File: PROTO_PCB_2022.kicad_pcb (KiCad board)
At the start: 2 copper layers, 86.4 x 49.5 mm, 15 parts, among them J1 ECU_EN_CONNECTON_1, J2 SMALL_12V_BATTERY_CONNECTOR, J3 12V_EXTRA, J4 ECU_EN_CONECTION_2, J5 ECU_EN_CONECTION_3, K2 RT214012, Q1 HORN_MOSFET1, Q2 BRAKELIGHTS_MOSFET1

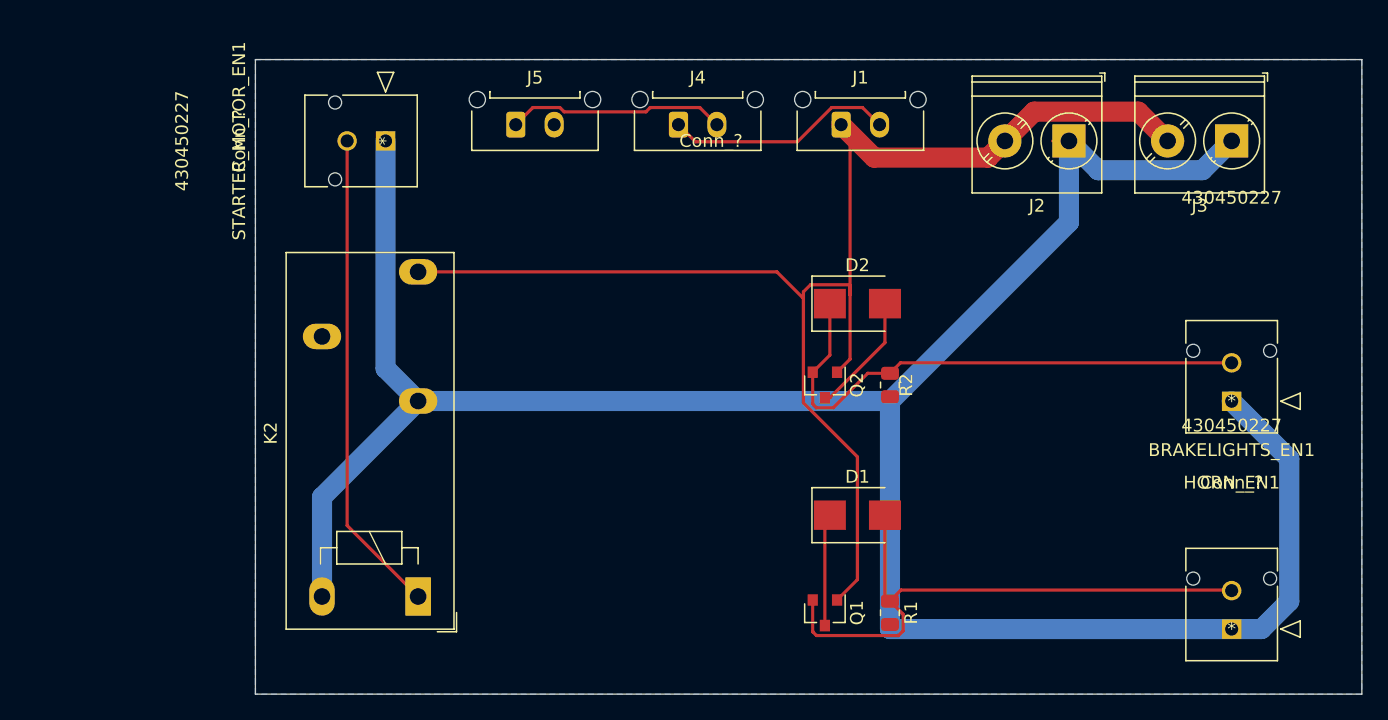
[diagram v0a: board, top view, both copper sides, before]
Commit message: Draft PCB for Report Purposes
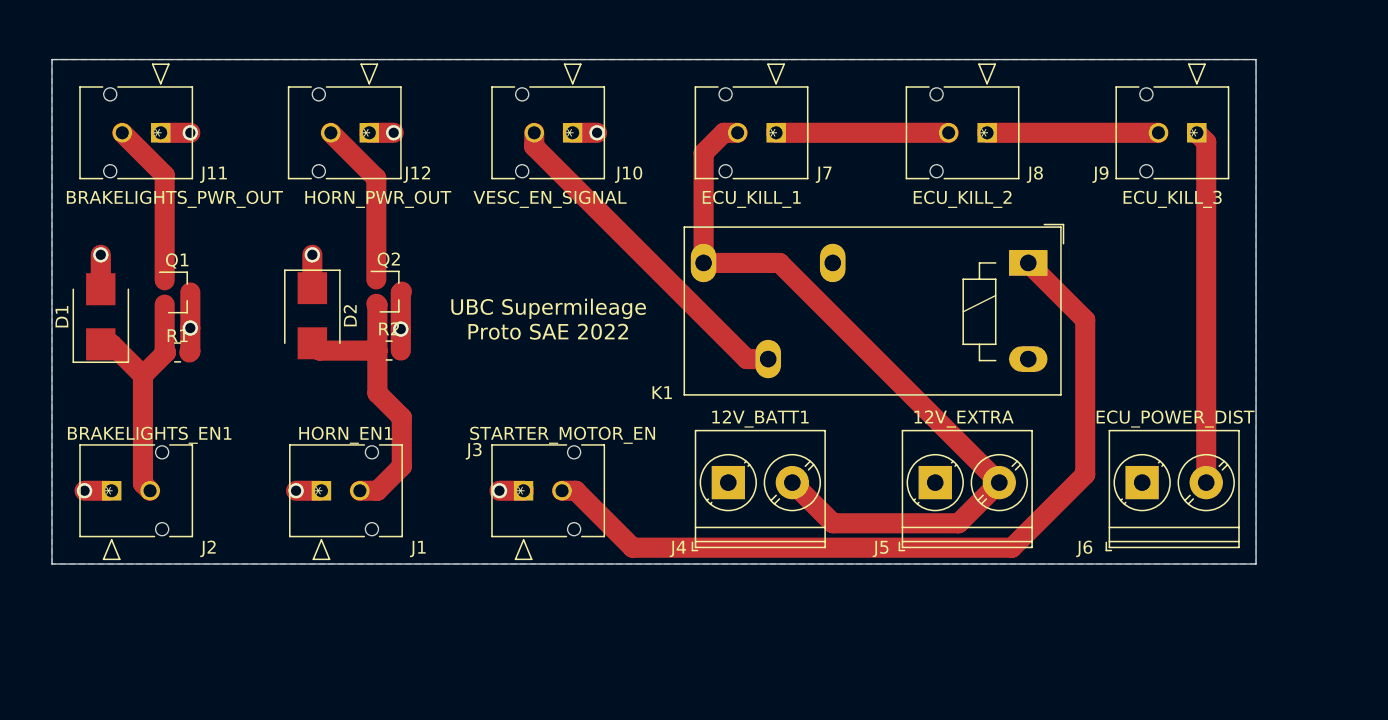
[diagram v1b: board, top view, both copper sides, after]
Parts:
- removed the J1 at (133.3, 83.8)
- removed the J4 at (120.7, 83.8)
- removed the J5 at (108.0, 83.8)
- added J10: VESC_EN_SIGNAL, Footprint Library:Molex_Proto_Microfit_Footprint, F.Cu at (112.4, 84.5)
- added J11: BRAKELIGHTS_PWR_OUT, Footprint Library:Molex_Proto_Microfit_Footprint, F.Cu at (80.2, 84.5)
- added J12: HORN_PWR_OUT, Footprint Library:Molex_Proto_Microfit_Footprint, F.Cu at (96.5, 84.5)
- added J6: ECU_POWER_DIST, TerminalBlock_Phoenix:TerminalBlock_Phoenix_PT-1,5-2-5.0-H_1x02_P5.00mm_Horizontal, F.Cu at (156.8, 111.8)
- added J7: ECU_KILL_1, Footprint Library:Molex_Proto_Microfit_Footprint, F.Cu at (128.3, 84.5)
- added J8: ECU_KILL_2, Footprint Library:Molex_Proto_Microfit_Footprint, F.Cu at (144.7, 84.5)
- added J9: ECU_KILL_3, Footprint Library:Molex_Proto_Microfit_Footprint, F.Cu at (161.1, 84.5)
- D1: renamed from D2; value BRAKELIGHTS_D_TVS -> (none)
- D2: renamed from D1; value HORN_D_TVS -> (none)
- J1: renamed from HORN_EN1; value Conn_? -> HORN_EN1
- J2: renamed from BRAKELIGHTS_EN1; value Conn_? -> BRAKELIGHTS_EN1
- J3: renamed from STARTER_MOTOR_EN1; value Conn_? -> STARTER_MOTOR_EN
- J4: renamed from J2; value SMALL_12V_BATTERY_CONNECTOR -> 12V_BATT1
- K1: renamed from K2; value RT214012 -> (none)
- Q1: renamed from Q2; value BRAKELIGHTS_MOSFET1 -> (none)
- Q2: renamed from Q1; value HORN_MOSFET1 -> (none)
- R1: renamed from R2; value 10k -> (none)
- R2: renamed from R1; value 10k -> (none)
- moved J2 87.7 mm to (76.4, 112.4), turned to 270 degrees
- moved J1 71.9 mm to (92.8, 112.4), turned to 270 degrees
- moved D1 59.1 mm to (75.6, 98.8), turned to 90 degrees
- moved R1 55.7 mm to (81.6, 101.6), turned to 0 degrees
- moved K1 54.3 mm to (148.0, 94.6), turned to 180 degrees
- moved Q1 51.0 mm to (81.5, 96.9), turned to 0 degrees
- moved D2 45.3 mm to (92.1, 98.7), turned to 270 degrees
- moved R2 44.1 mm to (98.1, 101.5), turned to 0 degrees
- moved Q2 42.3 mm to (98.1, 96.9), turned to 0 degrees
- moved J4 37.7 mm to (124.5, 111.8), turned to 0 degrees
- moved J5 35.3 mm to (140.7, 111.8), turned to 0 degrees
- moved J3 29.4 mm to (108.6, 112.4), turned to 270 degrees
- renumbered J3 to J5
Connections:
- D1 pad 2: BRAKELIGHTS_PWR -> GND
- D2 pad 1: HORN_PWR -> GND
- K1 pad 11: VESC_POWER_CONNECTION -> VESC_EN_SIGNAL
- Q1 pad 1: ECU_KILL_EN_TOGGLESWITCH_1A -> BRAKELIGHTS_PWR_OUT
- Q1 pad 3: BRAKELIGHTS_PWR -> GND
- Q2 pad 1: ECU_KILL_EN_TOGGLESWITCH_1A -> HORN_PWR_OUT
- Q2 pad 3: HORN_PWR -> GND
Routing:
- net GND: track 184.7 -> 26.5 mm, vias 0 -> 10
- net ECU_KILL_EN_TOGGLESWITCH_1A: track 111.0 -> 60.9 mm
- net ECU_KILL_EN_TOGGLESWITCH_3B: track 0.00 -> 27.6 mm
- net VESC_EN_SIGNAL: track 0.00 -> 26.2 mm
- net STARTER_EN_PUSHBUTTON: track 37.9 -> 63.4 mm
- net HORN_EN_12V_SIGNAL: track 46.5 -> 23.4 mm
- net BRAKELIGHTS_EN_12V_SIGNAL: track 42.7 -> 19.8 mm
- net HORN_PWR_OUT: track 0.00 -> 12.9 mm
- net BRAKELIGHTS_PWR_OUT: track 0.00 -> 12.9 mm
- net BRAKELIGHTS_PWR: track 9.52 -> 0.00 mm
- net HORN_PWR: track 8.78 -> 0.00 mm
- net ECU_KILL_EN_TOGGLESWITCH_1B: track 17.9 -> 13.5 mm
- net ECU_KILL_EN_TOGGLESWITCH_2B: track 17.1 -> 13.4 mm
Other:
- board size 86.4 x 49.5 mm -> 94 x 39.4 mm
- board text added: "UBC Supermileage Proto SAE 2022"

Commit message: second version
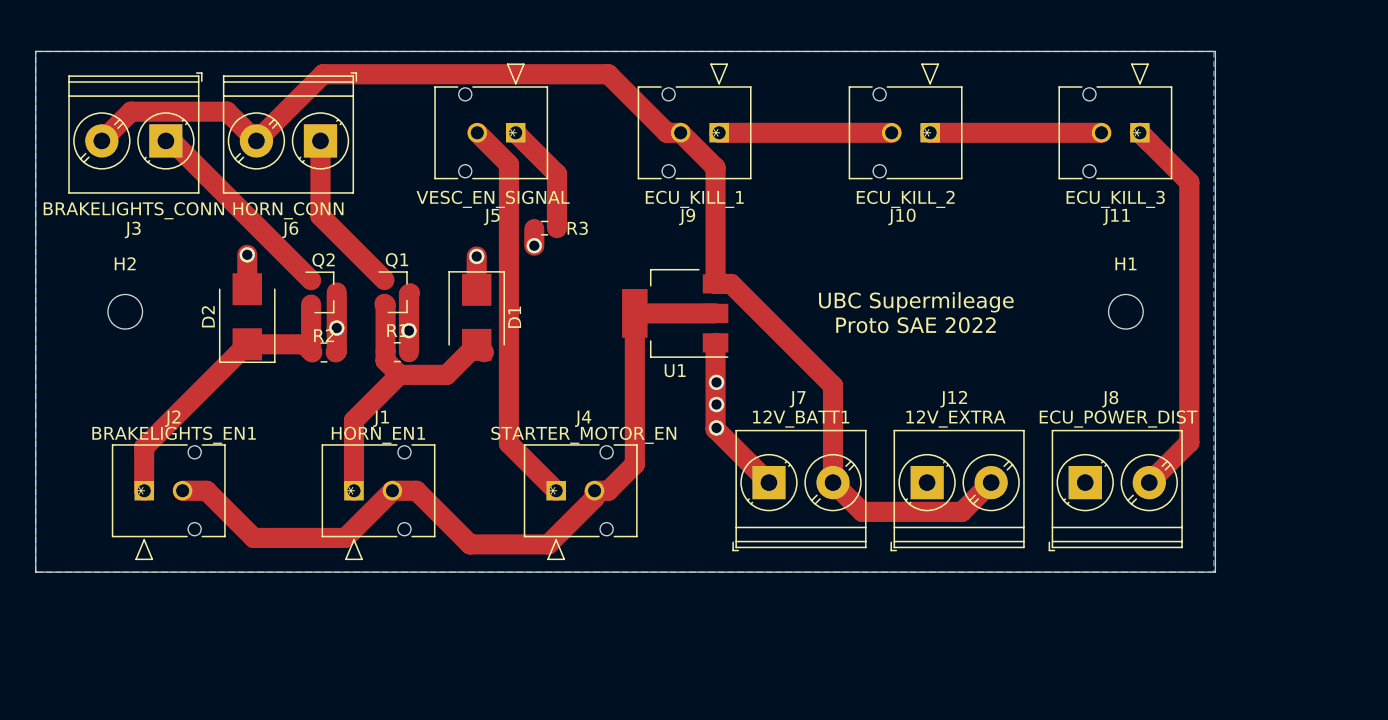
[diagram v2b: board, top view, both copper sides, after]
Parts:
- removed the J11 at (80.2, 84.5)
- removed the J12 at (96.5, 84.5)
- removed K1: , Relay_THT:Relay_SPDT_Schrack-RT1-FormC_RM5mm
- added H1: MountingHole, MountingHole:MountingHole_2.7mm_M2.5, F.Cu at (155.6, 98.4)
- added H2: MountingHole, MountingHole:MountingHole_2.7mm_M2.5, F.Cu at (77.5, 98.4)
- added J3: BRAKELIGHTS_CONN, TerminalBlock_Phoenix:TerminalBlock_Phoenix_PT-1,5-2-5.0-H_1x02_P5.00mm_Horizontal, F.Cu at (80.6, 85.1)
- added J6: HORN_CONN, TerminalBlock_Phoenix:TerminalBlock_Phoenix_PT-1,5-2-5.0-H_1x02_P5.00mm_Horizontal, F.Cu at (92.7, 85.1)
- added R3: , Resistor_SMD:R_0603_1608Metric, F.Cu at (110.2, 91.9)
- added U1: , Package_TO_SOT_SMD:SOT-223-3_TabPin2, F.Cu at (120.4, 98.6)
- R1: renamed from R2; value (none) -> 10k
- moved D1 12.8 mm to (104.9, 98.9)
- moved D2 11.4 mm to (87.0, 98.8)
- moved Q2 11.4 mm to (93.0, 96.9)
- moved R2 11.4 mm to (93.0, 101.6)
- moved J10 4.45 mm to (140.3, 84.5)
- moved J11 4.45 mm to (156.7, 84.5)
- moved J9 4.45 mm to (123.8, 84.5)
- moved J5 4.44 mm to (108.0, 84.5)
- moved J8 4.44 mm to (152.4, 111.8)
- moved J7 3.17 mm to (127.7, 111.8)
- moved J1 2.54 mm to (95.3, 112.4)
- moved J2 2.54 mm to (79.0, 112.4)
- moved J4 2.54 mm to (111.1, 112.4)
- moved R1 0.65 mm to (98.7, 101.6)
- moved Q1 0.64 mm to (98.7, 96.9)
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- renumbered D2 to D1, D1 to D2, J8 to J10, J9 to J11, J5 to J12, J3 to J4, J10 to J5, J4 to J7, J6 to J8, J7 to J9, Q2 to Q1, Q1 to Q2, R1 to R2
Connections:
- net ECU_KILL_EN_TOGGLESWITCH_1A renamed 12V_FOR_BRAKELIGHTS
- D1 pad 2: HORN_EN_12V_SIGNAL -> HORN_EN_5V
- D2 pad 1: BRAKELIGHTS_EN_12V_SIGNAL -> BRAKELIGHTS_EN_5V
- J1 pad 1: GND -> HORN_EN_5V
- J1 pad 2: HORN_EN_12V_SIGNAL -> +5V
- J2 pad 1: GND -> BRAKELIGHTS_EN_5V
- J2 pad 2: BRAKELIGHTS_EN_12V_SIGNAL -> +5V
- J4 pad 1: GND -> VESC_EN_5V
- J4 pad 2: STARTER_EN_PUSHBUTTON -> +5V
- J5 pad 1: GND -> Net-(J5-Pad1)
- J5 pad 2: VESC_EN_SIGNAL -> VESC_EN_5V
- Q1 pad 1: HORN_PWR_OUT -> HORN_GND
- Q1 pad 2: HORN_EN_12V_SIGNAL -> HORN_EN_5V
- Q2 pad 1: BRAKELIGHTS_PWR_OUT -> BRAKELIGHTS_GND
- Q2 pad 2: BRAKELIGHTS_EN_12V_SIGNAL -> BRAKELIGHTS_EN_5V
- R1 pad 1: HORN_EN_12V_SIGNAL -> HORN_EN_5V
- R2 pad 1: BRAKELIGHTS_EN_12V_SIGNAL -> BRAKELIGHTS_EN_5V
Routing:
- net STARTER_EN_PUSHBUTTON: track 63.4 -> 0.00 mm
- net +5V: track 0.00 -> 61.1 mm
- net 12V_FOR_BRAKELIGHTS: track 60.9 -> 98.3 mm
- net VESC_EN_5V: track 0.00 -> 30.5 mm
- net VESC_EN_SIGNAL: track 26.2 -> 0.00 mm
- net HORN_EN_5V: track 0.00 -> 24.8 mm
- net BRAKELIGHTS_EN_5V: track 0.00 -> 24.6 mm
- net HORN_EN_12V_SIGNAL: track 23.4 -> 0.00 mm
- net BRAKELIGHTS_EN_12V_SIGNAL: track 19.8 -> 0.00 mm
- net BRAKELIGHTS_GND: track 0.00 -> 15.8 mm
- net HORN_GND: track 0.00 -> 12.9 mm
- net HORN_PWR_OUT: track 12.9 -> 0.00 mm
- net BRAKELIGHTS_PWR_OUT: track 12.9 -> 0.00 mm
- net Net-(J5-Pad1): track 0.00 -> 8.78 mm
- net ECU_KILL_EN_TOGGLESWITCH_3B: track 27.6 -> 31.2 mm
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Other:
- board size 94 x 39.4 mm -> 92.1 x 40.6 mm
